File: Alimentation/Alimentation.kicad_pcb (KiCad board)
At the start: 2 copper layers, 72.4 x 85 mm, 18 parts, among them J1 RPI, J10 BATTERY PARACHUTE, J11 STEPPER_VOUT, J12 SWITCH_RPI, J13 SWITCH_PARA, J14 SWITCH_LORA, J2 STEPPER, J3 LORA, J4 BATTERY RPI EXPE, J5 BATTERY LORA, J6 RPI_VOUT, J7 STEPPER_VOUT, J8 LORA_VOUT, J9 PARACHUTE

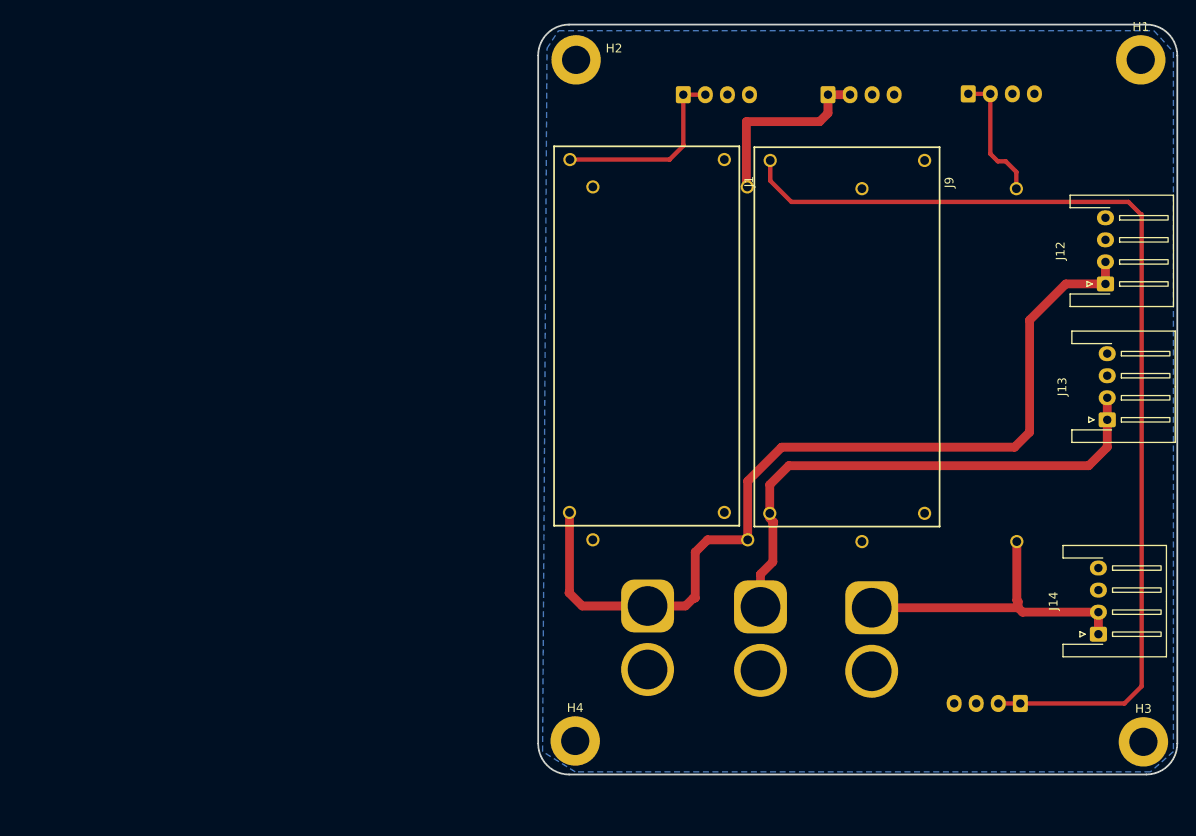
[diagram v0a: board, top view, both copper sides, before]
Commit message: alimentation: full revision
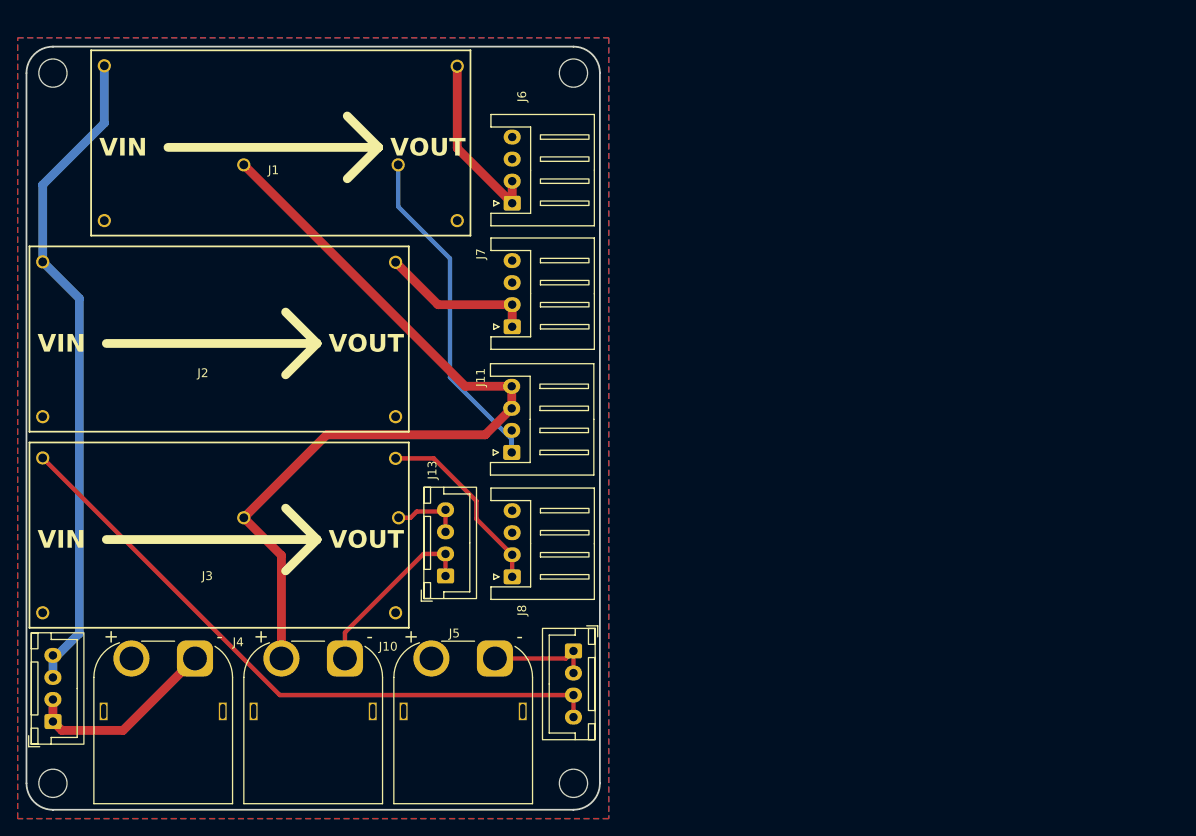
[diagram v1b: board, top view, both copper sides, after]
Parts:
- removed H3, H4: MountingHole_Pad, MountingHole:MountingHole_3.2mm_M3_DIN965_Pad
- added H5: MountingHole_3.2mm_M3, MountingHole:MountingHole_3.2mm_M3, F.Cu at (61.0, 130.5)
- added H6: MountingHole_3.2mm_M3, MountingHole:MountingHole_3.2mm_M3, F.Cu at (120.0, 130.5)
- H1, H2: value MountingHole_Pad -> MountingHole_3.2mm_M3; footprint MountingHole:MountingHole_3.2mm_M3_DIN965_Pad -> MountingHole:MountingHole_3.2mm_M3
- J1: footprint PHOENIX:BUCK_STEPDOWN_LM2592 -> nasa:LM2596
- J10, J4, J5: footprint PHOENIX_CON:AMASS_XT60-M_1x02_P7.20mm_Vertical -> Connector_AMASS:AMASS_XT60PW-M_1x02_P7.20mm_Horizontal; moved to F.Cu
- J11: value STEPPER_VOUT -> PARACHUTE_VOUT; footprint Connector_JST:JST_XH_S4B-XH-A-1_1x04_P2.50mm_Horizontal -> Connector_JST:JST_XH_S4B-XH-A_1x04_P2.50mm_Horizontal; moved to F.Cu
- J12, J13, J14: footprint Connector_JST:JST_XH_S4B-XH-A-1_1x04_P2.50mm_Horizontal -> Connector_JST:JST_XH_B4B-XH-A_1x04_P2.50mm_Vertical
- J2, J3: footprint PHOENIX:BUCK_STEPDOWN_LM2592 -> nasa:LM2596; moved to F.Cu
- J6, J7, J8: footprint Connector_JST:JST_XH_S4B-XH-A-1_1x04_P2.50mm_Horizontal -> Connector_JST:JST_XH_S4B-XH-A_1x04_P2.50mm_Horizontal; moved to F.Cu
- J9: footprint PHOENIX:BUCK_STEPDOWN_LM2592 -> nasa:LM2596; moved to B.Cu
- moved J12 129.2 mm to (61.0, 123.5)
- moved H1 123.3 mm to (61.0, 50.0)
- moved J3 84.4 mm to (78.7, 102.9), turned to 0 degrees
- moved J13 77.1 mm to (105.5, 107.0)
- moved J8 75.3 mm to (113.1, 107.1), turned to 90 degrees
- moved J11 64.3 mm to (113.0, 93.0), turned to 90 degrees
- moved J9 60.6 mm to (90.9, 81.5)
- moved J14 59.5 mm to (120.0, 115.5), turned to -90 degrees
- moved J2 51.9 mm to (78.7, 80.6), turned to 0 degrees
- moved J4 51.6 mm to (77.1, 116.3), turned to 180 degrees
- moved J1 48.6 mm to (85.7, 58.4), turned to 0 degrees
- moved J10 47.5 mm to (94.1, 116.3), turned to 180 degrees
- moved J7 44.4 mm to (113.1, 78.8), turned to 90 degrees
- moved J5 43.1 mm to (111.1, 116.3), turned to 180 degrees
- moved J6 23.0 mm to (113.1, 64.8), turned to 90 degrees
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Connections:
- J1 pad 1: +VIN_RPI -> +VCC_RPI
- J10 pad 2: GND -> GND1
- J11 pad 3: GND -> GND1
- J11 pad 4: GND -> GND1
- J12 pad 3: GND -> +VCC_RPI
- J12 pad 4: GND -> +VCC_RPI
- J13 pad 3: GND -> +VCC_PARA
- J13 pad 4: GND -> +VCC_PARA
- J14 pad 3: GND -> +VCC_LORA
- J14 pad 4: GND -> +VCC_LORA
- J2 pad 1: +VIN_RPI -> +VCC_RPI
- J3 pad 1: +VIN_LORA -> +VCC_LORA
- J9 pad 1: +VIN_PARA -> +VCC_PARA
- J9 pad 3: GND -> GND1
- J9 pad 4: GND -> GND1
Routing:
- net GND1: track 0.00 -> 96.5 mm
- net +VIN_RPI: track 102.5 -> 22.4 mm
- net +5V_PARA: track 116.4 -> 40.4 mm
- net +VCC_RPI: track 0.00 -> 75.5 mm
- net +VCC_LORA: track 0.00 -> 73.8 mm
- net +VIN_PARA: track 60.3 -> 20.5 mm
- net +VIN_LORA: track 36.0 -> 11.8 mm
- net +VCC_PARA: track 0.00 -> 8.19 mm
- net +3V3_LORA: track 15.0 -> 21.4 mm
- net +VOUT_STEPPER: track 21.7 -> 17.7 mm
- net +5V_RPI: track 21.8 -> 20.6 mm
- added copper zone on F.Cu, net GND
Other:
- board size 72.4 x 85 mm -> 65 x 86.5 mm
- board text added: "BATTERY"
- board text added: "LORA"
- board text added: "PARACHUTE"
- board text added: "RASPI"
- board text added: "STEPPER"
- board text added: "SW LORA"
- board text added: "SW PARACHUTE"
- board text added: "SW RASPI"
